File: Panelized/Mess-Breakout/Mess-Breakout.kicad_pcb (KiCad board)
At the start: 2 copper layers, 99.8 x 99.5 mm, 165 parts, among them J10 Conn_01x30_Pin, J11 Conn_02x30_Odd_Even, J2 Conn_01x30_Pin, J3 Conn_01x30_Pin, J4 Conn_01x30_Pin, J5 Conn_02x30_Odd_Even, J6 Conn_02x30_Odd_Even, J7 Conn_02x30_Odd_Even, J8 Conn_01x30_Pin, J9 Conn_02x30_Odd_Even, P1 Jumper4x1, P10 Jumper4x1, P100 Jumper4x1, P101 Jumper4x1, P102 Jumper4x1, P103 Jumper4x1, P104 Jumper4x1, P105 Jumper4x1, P106 Jumper4x1, P107 Jumper4x1, P108 Jumper4x1, P109 Jumper4x1, P11 Jumper4x1, P110 Jumper4x1, P111 Jumper4x1, P112 Jumper4x1, P113 Jumper4x1, P114 Jumper4x1, P115 Jumper4x1, P116 Jumper4x1, P117 Jumper4x1, P118 Jumper4x1, P119 Jumper4x1, P12 Jumper4x1, P120 Jumper4x1, P121 Jumper4x1, P122 Jumper4x1, P123 Jumper4x1, P124 Jumper4x1, P125 Jumper4x1, P126 Jumper4x1, P127 Jumper4x1, P128 Jumper4x1, P129 Jumper4x1, P13 Jumper4x1, P130 Jumper4x1, P131 Jumper4x1, P132 Jumper4x1, P133 Jumper4x1, P134 Jumper4x1, P135 Jumper4x1, P136 Jumper4x1, P137 Jumper4x1, P138 Jumper4x1, P139 Jumper4x1, P14 Jumper4x1, P140 Jumper4x1, P141 Jumper4x1, P142 Jumper4x1, P143 Jumper4x1, P144 Jumper4x1, P145 Jumper4x1, P146 Jumper4x1, P147 Jumper4x1, P148 Jumper4x1, P149 Jumper4x1, P15 Jumper4x1, P150 Jumper4x1, P16 Jumper4x1, P17 Jumper4x1, P18 Jumper4x1, P19 Jumper4x1, P2 Jumper4x1, P20 Jumper4x1, P21 Jumper4x1, P22 Jumper4x1, P23 Jumper4x1, P24 Jumper4x1, P25 Jumper4x1, P26 Jumper4x1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

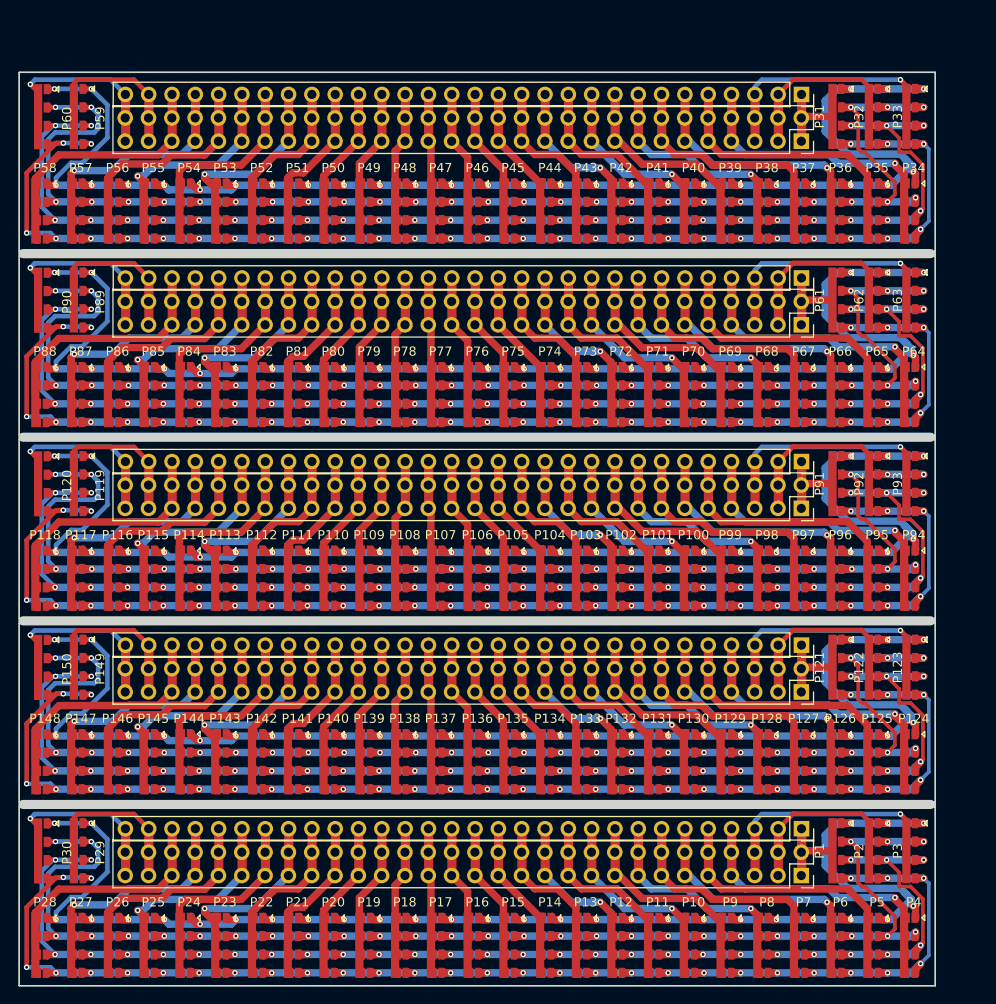
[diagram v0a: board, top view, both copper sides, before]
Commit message: update.
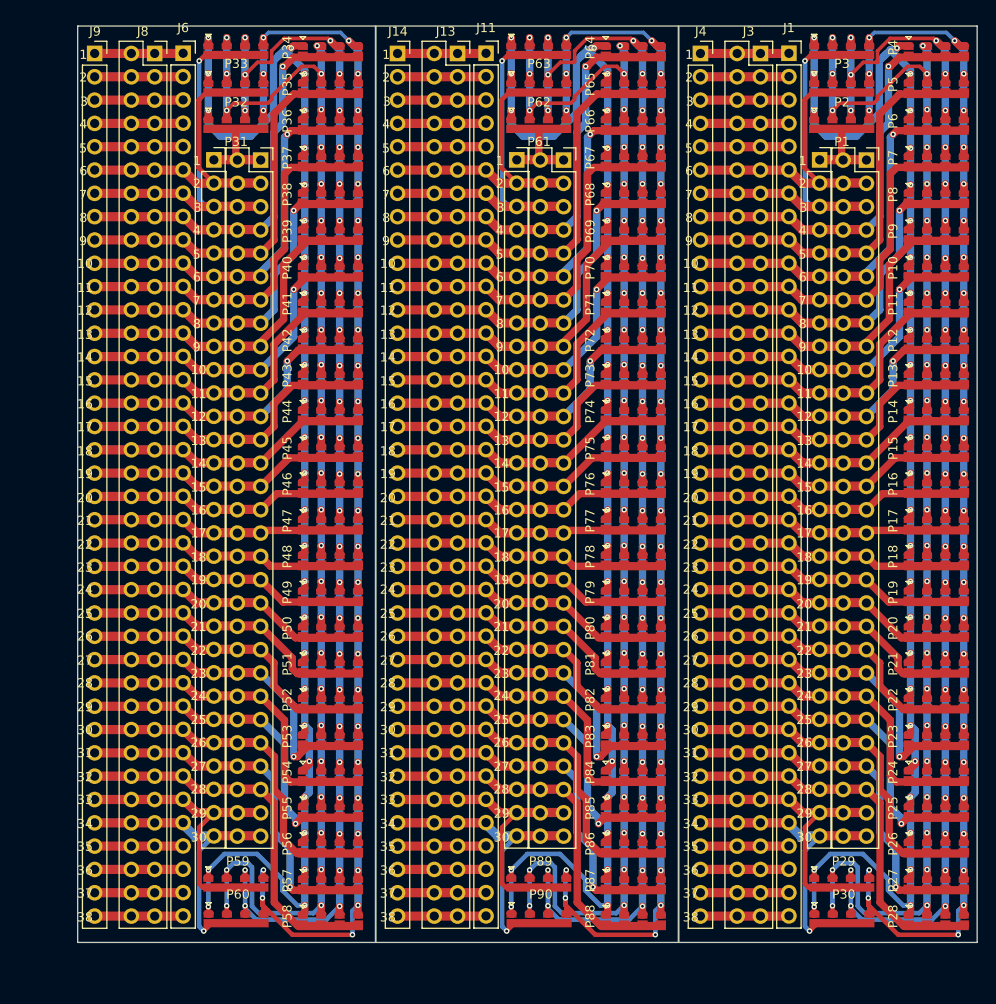
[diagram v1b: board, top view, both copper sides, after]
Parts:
- removed G***3, G***4: LOGO, IOT-Mess-Footprints:catIcon8x8
- removed P100, P101, P102, P103, P104, P105, P106, P107, P108, P109, P110, P111, P112, P113, P114, P115, P116, P117, P118, P119, P120, P121, P122, P123, P124, P125, P126, P127, P128, P129, P130, P131, P132, P133, P134, P135, P136, P137, P138, P139, P140, P141, P142, P143, P144, P145, P146, P147, P148, P149, P150, P91, P92, P93, P94, P95, P96, P97, P98, P99: Jumper4x1, IOT-Mess-Footprints:Jumper4x1
- added J1: Conn_01x38_Pin, Connector_PinSocket_2.54mm:PinSocket_1x38_P2.54mm_Vertical, F.Cu at (152.7, 52.3)
- added J12: Conn_01x30_Pin, Connector_PinSocket_2.54mm:PinSocket_1x30_P2.54mm_Vertical, F.Cu at (123.0, 63.9)
- added J13: Conn_02x38_Odd_Even, Connector_PinSocket_2.54mm:PinSocket_2x38_P2.54mm_Vertical, F.Cu at (116.6, 52.3)
- added J14: Conn_01x38_Pin, Connector_PinSocket_2.54mm:PinSocket_1x38_P2.54mm_Vertical, F.Cu at (110.0, 52.3)
- added J15: Conn_02x30_Odd_Even, Connector_PinSocket_2.54mm:PinSocket_2x30_P2.54mm_Vertical, F.Cu at (128.1, 64.0)
- J10: value Conn_01x30_Pin -> Conn_02x30_Odd_Even; footprint Connector_PinSocket_2.54mm:PinSocket_1x30_P2.54mm_Vertical -> Connector_PinSocket_2.54mm:PinSocket_2x30_P2.54mm_Vertical
- J11, J6, J9: value Conn_02x30_Odd_Even -> Conn_01x38_Pin; footprint Connector_PinSocket_2.54mm:PinSocket_2x30_P2.54mm_Vertical -> Connector_PinSocket_2.54mm:PinSocket_1x38_P2.54mm_Vertical
- J3, J8: value Conn_01x30_Pin -> Conn_02x38_Odd_Even; footprint Connector_PinSocket_2.54mm:PinSocket_1x30_P2.54mm_Vertical -> Connector_PinSocket_2.54mm:PinSocket_2x38_P2.54mm_Vertical
- J4: value Conn_01x30_Pin -> Conn_01x38_Pin; footprint Connector_PinSocket_2.54mm:PinSocket_1x30_P2.54mm_Vertical -> Connector_PinSocket_2.54mm:PinSocket_1x38_P2.54mm_Vertical
- J7: value Conn_02x30_Odd_Even -> Conn_01x30_Pin; footprint Connector_PinSocket_2.54mm:PinSocket_2x30_P2.54mm_Vertical -> Connector_PinSocket_2.54mm:PinSocket_1x30_P2.54mm_Vertical
- moved P28 95.2 mm to (165.7, 147.4), turned to 90 degrees
- moved P4 93.8 mm to (165.7, 52.8), turned to 90 degrees
- moved P60 92.8 mm to (89.4, 147.1), turned to 90 degrees
- moved J9 91.6 mm to (77.0, 52.3), turned to 0 degrees
- moved P27 91.3 mm to (165.7, 143.5), turned to 90 degrees
- moved P5 89.9 mm to (165.7, 56.8), turned to 90 degrees
- moved P59 88.2 mm to (89.4, 143.2), turned to 90 degrees
- moved P90 87.7 mm to (122.4, 147.1), turned to 90 degrees
- moved P26 87.5 mm to (165.7, 139.5), turned to 90 degrees
- moved P88 87.0 mm to (132.7, 147.4), turned to 90 degrees
- moved P6 86.2 mm to (165.7, 60.8), turned to 90 degrees
- moved P58 86.0 mm to (99.7, 147.4), turned to 90 degrees
- moved P30 85.3 mm to (155.4, 147.1), turned to 90 degrees
- moved P3 84.3 mm to (155.4, 52.5), turned to 90 degrees
- moved P25 84.1 mm to (165.7, 135.6), turned to 90 degrees
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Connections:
- J10 pad 10: P10 -> P5
- J10 pad 11: P11 -> P6
- J10 pad 12: P12 -> P6
- J10 pad 13: P13 -> P7
- J10 pad 14: P14 -> P7
- J10 pad 15: P15 -> P8
- J10 pad 16: P16 -> P8
- J10 pad 17: P17 -> P9
- J10 pad 18: P18 -> P9
- J10 pad 19: P19 -> P10
- J10 pad 2: P2 -> P1
- J10 pad 20: P20 -> P10
- J10 pad 21: P21 -> P11
- J10 pad 22: P22 -> P11
- J10 pad 23: P23 -> P12
- J10 pad 24: P24 -> P12
- J10 pad 25: P25 -> P13
- J10 pad 26: P26 -> P13
- J10 pad 27: P27 -> P14
- J10 pad 28: P28 -> P14
- J10 pad 29: P29 -> P15
- J10 pad 3: P3 -> P2
- J10 pad 30: P30 -> P15
- J10 pad 4: P4 -> P2
- J10 pad 5: P5 -> P3
- J10 pad 6: P6 -> P3
- J10 pad 7: P7 -> P4
- J10 pad 8: P8 -> P4
- J10 pad 9: P9 -> P5
- J11 pad 1: P1 -> /B1
- J11 pad 10: P5 -> P6
- J11 pad 11: P6 -> P7
- J11 pad 12: P6 -> P8
- J11 pad 13: P7 -> P9
- J11 pad 14: P7 -> P10
- J11 pad 15: P8 -> P11
- J11 pad 16: P8 -> P12
- J11 pad 17: P9 -> P13
- J11 pad 18: P9 -> P14
- J11 pad 19: P10 -> P15
- J11 pad 2: P1 -> /B2
- J11 pad 20: P10 -> P16
- J11 pad 21: P11 -> P17
- J11 pad 22: P11 -> P18
- J11 pad 23: P12 -> P19
- J11 pad 24: P12 -> P20
- J11 pad 25: P13 -> P21
- J11 pad 26: P13 -> P22
- J11 pad 27: P14 -> P23
- J11 pad 28: P14 -> P24
- J11 pad 29: P15 -> P25
- J11 pad 3: P2 -> /B3
- J11 pad 30: P15 -> P26
- J11 pad 31: P16 -> P27
- J11 pad 32: P16 -> P28
- J11 pad 33: P17 -> P29
- J11 pad 34: P17 -> P30
- J11 pad 35: P18 -> /B35
- J11 pad 36: P18 -> /B36
- J11 pad 37: P19 -> /B37
- J11 pad 38: P19 -> /B38
- J11 pad 4: P2 -> /B4
- J11 pad 5: P3 -> /B5
- J11 pad 6: P3 -> P2
- J11 pad 7: P4 -> P3
- J3 pad 1: P1 -> /B1
- J3 pad 10: P10 -> /B5
- J3 pad 11: P11 -> P2
- J3 pad 12: P12 -> P2
- J3 pad 13: P13 -> P3
- J3 pad 14: P14 -> P3
- J3 pad 15: P15 -> P4
- J3 pad 16: P16 -> P4
- J3 pad 17: P17 -> P5
- J3 pad 18: P18 -> P5
- J3 pad 19: P19 -> P6
- J3 pad 2: P2 -> /B1
- J3 pad 20: P20 -> P6
- J3 pad 21: P21 -> P7
- J3 pad 22: P22 -> P7
- J3 pad 23: P23 -> P8
- J3 pad 24: P24 -> P8
- J3 pad 25: P25 -> P9
- J3 pad 26: P26 -> P9
- J3 pad 27: P27 -> P10
- J3 pad 28: P28 -> P10
- J3 pad 29: P29 -> P11
- J3 pad 3: P3 -> /B2
- J3 pad 30: P30 -> P11
- J3 pad 4: P4 -> /B2
- J3 pad 5: P5 -> /B3
- J3 pad 6: P6 -> /B3
- J3 pad 7: P7 -> /B4
- J3 pad 8: P8 -> /B4
- J3 pad 9: P9 -> /B5
- J4 pad 1: P1 -> /B1
- J4 pad 10: P10 -> P6
- J4 pad 11: P11 -> P7
- J4 pad 12: P12 -> P8
- J4 pad 13: P13 -> P9
- J4 pad 14: P14 -> P10
- J4 pad 15: P15 -> P11
- J4 pad 16: P16 -> P12
- J4 pad 17: P17 -> P13
- J4 pad 18: P18 -> P14
- J4 pad 19: P19 -> P15
- J4 pad 2: P2 -> /B2
- J4 pad 20: P20 -> P16
- J4 pad 21: P21 -> P17
- J4 pad 22: P22 -> P18
- J4 pad 23: P23 -> P19
- J4 pad 24: P24 -> P20
- J4 pad 25: P25 -> P21
- J4 pad 26: P26 -> P22
- J4 pad 27: P27 -> P23
- J4 pad 28: P28 -> P24
- J4 pad 29: P29 -> P25
- J4 pad 3: P3 -> /B3
- J4 pad 30: P30 -> P26
- J4 pad 4: P4 -> /B4
- J4 pad 5: P5 -> /B5
- J4 pad 6: P6 -> P2
- J4 pad 7: P7 -> P3
- J4 pad 8: P8 -> P4
- J4 pad 9: P9 -> P5
- J6 pad 1: P1 -> /B1
- J6 pad 10: P5 -> P6
- J6 pad 11: P6 -> P7
- J6 pad 12: P6 -> P8
- J6 pad 13: P7 -> P9
- J6 pad 14: P7 -> P10
- J6 pad 15: P8 -> P11
- J6 pad 16: P8 -> P12
- J6 pad 17: P9 -> P13
- J6 pad 18: P9 -> P14
- J6 pad 19: P10 -> P15
- J6 pad 2: P1 -> /B2
- J6 pad 20: P10 -> P16
- J6 pad 21: P11 -> P17
- J6 pad 22: P11 -> P18
- J6 pad 23: P12 -> P19
- J6 pad 24: P12 -> P20
- J6 pad 25: P13 -> P21
- J6 pad 26: P13 -> P22
- J6 pad 27: P14 -> P23
- J6 pad 28: P14 -> P24
- J6 pad 29: P15 -> P25
- J6 pad 3: P2 -> /B3
- J6 pad 30: P15 -> P26
- J6 pad 31: P16 -> P27
- J6 pad 32: P16 -> P28
- J6 pad 33: P17 -> P29
- J6 pad 34: P17 -> P30
- J6 pad 35: P18 -> /B35
- J6 pad 36: P18 -> /B36
- J6 pad 37: P19 -> /B37
- J6 pad 38: P19 -> /B38
- J6 pad 4: P2 -> /B4
- J6 pad 5: P3 -> /B5
- J6 pad 6: P3 -> P2
- J6 pad 7: P4 -> P3
- J7 pad 10: P5 -> P10
- J7 pad 11: P6 -> P11
- J7 pad 12: P6 -> P12
- J7 pad 13: P7 -> P13
- J7 pad 14: P7 -> P14
- J7 pad 15: P8 -> P15
- J7 pad 16: P8 -> P16
- J7 pad 17: P9 -> P17
- J7 pad 18: P9 -> P18
- J7 pad 19: P10 -> P19
- J7 pad 2: P1 -> P2
- J7 pad 20: P10 -> P20
- J7 pad 21: P11 -> P21
- J7 pad 22: P11 -> P22
- J7 pad 23: P12 -> P23
- J7 pad 24: P12 -> P24
- J7 pad 25: P13 -> P25
- J7 pad 26: P13 -> P26
- J7 pad 27: P14 -> P27
- J7 pad 28: P14 -> P28
- J7 pad 29: P15 -> P29
- J7 pad 3: P2 -> P3
- J7 pad 30: P15 -> P30
- J7 pad 4: P2 -> P4
- J7 pad 5: P3 -> P5
- J7 pad 6: P3 -> P6
- J7 pad 7: P4 -> P7
- J7 pad 8: P4 -> P8
- J7 pad 9: P5 -> P9
- J8 pad 1: P1 -> /B1
- J8 pad 10: P10 -> /B5
- J8 pad 11: P11 -> P2
- J8 pad 12: P12 -> P2
- J8 pad 13: P13 -> P3
- J8 pad 14: P14 -> P3
- J8 pad 15: P15 -> P4
- J8 pad 16: P16 -> P4
- J8 pad 17: P17 -> P5
- J8 pad 18: P18 -> P5
- J8 pad 19: P19 -> P6
- J8 pad 2: P2 -> /B1
- J8 pad 20: P20 -> P6
- J8 pad 21: P21 -> P7
- J8 pad 22: P22 -> P7
- J8 pad 23: P23 -> P8
- J8 pad 24: P24 -> P8
- J8 pad 25: P25 -> P9
- J8 pad 26: P26 -> P9
- J8 pad 27: P27 -> P10
- J8 pad 28: P28 -> P10
- J8 pad 29: P29 -> P11
- J8 pad 3: P3 -> /B2
- J8 pad 30: P30 -> P11
- J8 pad 4: P4 -> /B2
- J8 pad 5: P5 -> /B3
- J8 pad 6: P6 -> /B3
- J8 pad 7: P7 -> /B4
- J8 pad 8: P8 -> /B4
- J8 pad 9: P9 -> /B5
- J9 pad 1: P1 -> /B1
- J9 pad 10: P5 -> P6
- J9 pad 11: P6 -> P7
- J9 pad 12: P6 -> P8
- J9 pad 13: P7 -> P9
- J9 pad 14: P7 -> P10
- J9 pad 15: P8 -> P11
- J9 pad 16: P8 -> P12
- J9 pad 17: P9 -> P13
- J9 pad 18: P9 -> P14
- J9 pad 19: P10 -> P15
- J9 pad 2: P1 -> /B2
- J9 pad 20: P10 -> P16
- J9 pad 21: P11 -> P17
- J9 pad 22: P11 -> P18
- J9 pad 23: P12 -> P19
- J9 pad 24: P12 -> P20
- J9 pad 25: P13 -> P21
- J9 pad 26: P13 -> P22
- J9 pad 27: P14 -> P23
- J9 pad 28: P14 -> P24
- J9 pad 29: P15 -> P25
- J9 pad 3: P2 -> /B3
- J9 pad 30: P15 -> P26
- J9 pad 31: P16 -> P27
- J9 pad 32: P16 -> P28
- J9 pad 33: P17 -> P29
- J9 pad 34: P17 -> P30
- J9 pad 35: P18 -> /B35
- J9 pad 36: P18 -> /B36
- J9 pad 37: P19 -> /B37
- J9 pad 38: P19 -> /B38
- J9 pad 4: P2 -> /B4
- J9 pad 5: P3 -> /B5
- J9 pad 6: P3 -> P2
- J9 pad 7: P4 -> P3
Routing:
- net /JA1: track 856.1 -> 513.6 mm, vias 150 -> 90
- net /JA2: track 815.2 -> 489.1 mm, vias 150 -> 90
- net /JA4: track 798.9 -> 479.4 mm, vias 155 -> 93
- net /JA3: track 788.6 -> 473.2 mm, vias 150 -> 90
- net /B38: track 0.00 -> 28.9 mm
- net /B37: track 0.00 -> 28.9 mm
- net /B35: track 0.00 -> 28.9 mm
- net /B5: track 0.00 -> 28.9 mm
- net /B4: track 0.00 -> 28.9 mm
- net /B3: track 0.00 -> 28.9 mm
- net /B2: track 0.00 -> 28.9 mm
- net /B1: track 0.00 -> 28.9 mm
- net /B36: track 0.00 -> 28.9 mm
- net P4: track 147.6 -> 129.3 mm, vias 5 -> 3
- net P1: track 42.7 -> 25.6 mm
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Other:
- board size 99.8 x 99.5 mm -> 98 x 99.8 mm
- board text added: "1"
- board text added: "10"
- board text added: "11"
- board text added: "12"
- board text added: "13"
- board text added: "14"
- board text added: "15"
- board text added: "16"
- board text added: "17"
- board text added: "18"
- board text added: "19"
- board text added: "2"
- board text added: "20"
- board text added: "21"
- board text added: "22"
- board text added: "23"
- board text added: "24"
- board text added: "25"
- board text added: "26"
- board text added: "27"
- board text added: "28"
- board text added: "29"
- board text added: "3"
- board text added: "30"
- board text added: "31"
- board text added: "32"
- board text added: "33"
- board text added: "34"
- board text added: "35"
- board text added: "36"
- board text added: "37"
- board text added: "38"
- board text added: "4"
- board text added: "5"
- board text added: "6"
- board text added: "7"
- board text added: "8"
- board text added: "9"
